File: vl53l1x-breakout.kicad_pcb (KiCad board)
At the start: 2 copper layers, 30 parts, among them J0 SM07B-SRSS-TBLFSN, J1 SM07B-SRSS-TBLFSN, U1 PCA9615DPJ, U2 VL53L1CXV0FY_1, U3 LTC4316IMSPBF

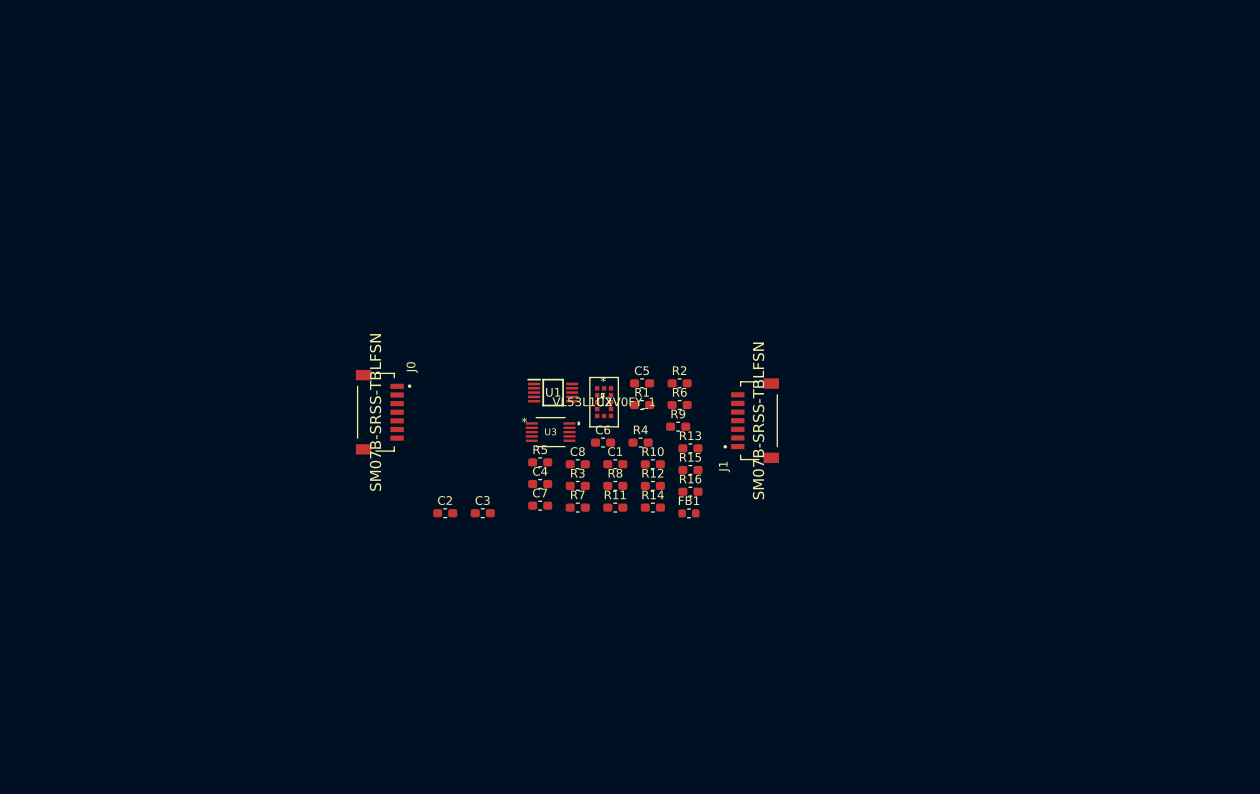
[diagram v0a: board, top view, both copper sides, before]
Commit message: [board] begin layout
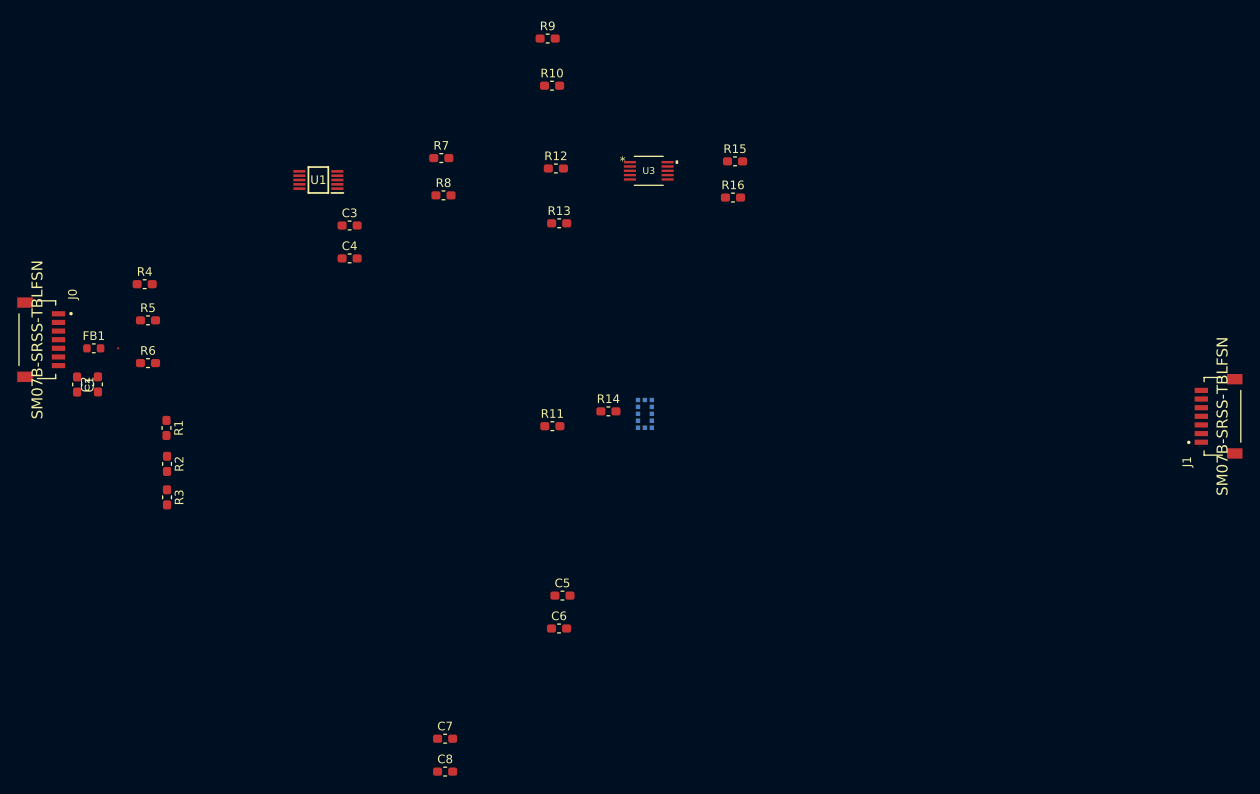
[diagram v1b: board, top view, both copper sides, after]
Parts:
- U2: moved to B.Cu
- moved FB1 71.5 mm to (107.0, 95.8)
- moved C1 63.0 mm to (105.1, 99.9), turned to 270 degrees
- moved R6 61.8 mm to (113.3, 97.5)
- moved R4 60.3 mm to (112.9, 88.3)
- moved R2 60.1 mm to (115.5, 109.1), turned to 270 degrees
- moved R1 55.1 mm to (115.4, 105.0), turned to 270 degrees
- moved J1 53.7 mm to (237.7, 103.6)
- moved R5 48.3 mm to (113.3, 92.5)
- moved R3 47.6 mm to (115.5, 113.0), turned to 270 degrees
- moved R9 47.4 mm to (159.6, 59.9)
- moved R10 45.4 mm to (160.1, 65.3)
- moved R7 43.5 mm to (147.3, 73.7)
- moved C2 42.9 mm to (107.5, 99.9), turned to 90 degrees
- moved J0 40.1 mm to (100.5, 94.8)
- moved R8 39.1 mm to (147.5, 78.0)
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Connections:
- J0 pad 1: SDA+ -> SCL-
- J0 pad 2: SDA- -> SCL+
- J0 pad 3: SCL+ -> SDA+
- J0 pad 4: SCL- -> SDA-
